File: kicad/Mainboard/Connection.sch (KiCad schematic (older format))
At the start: 12 parts, among them J12 GPS_CONN, J13 DBG_CONN, J15 Micro_SD_Card

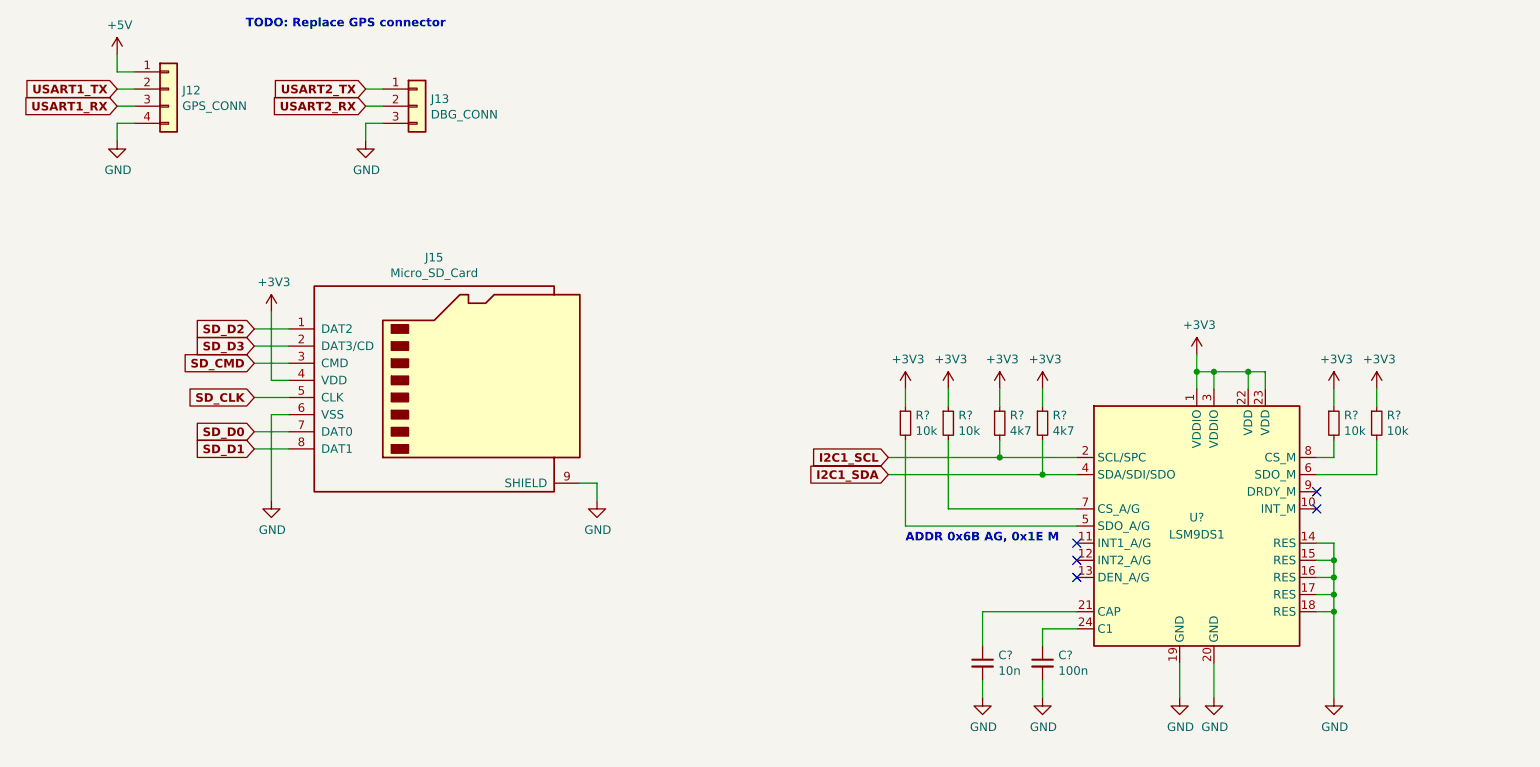
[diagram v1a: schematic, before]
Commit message: Add files via upload
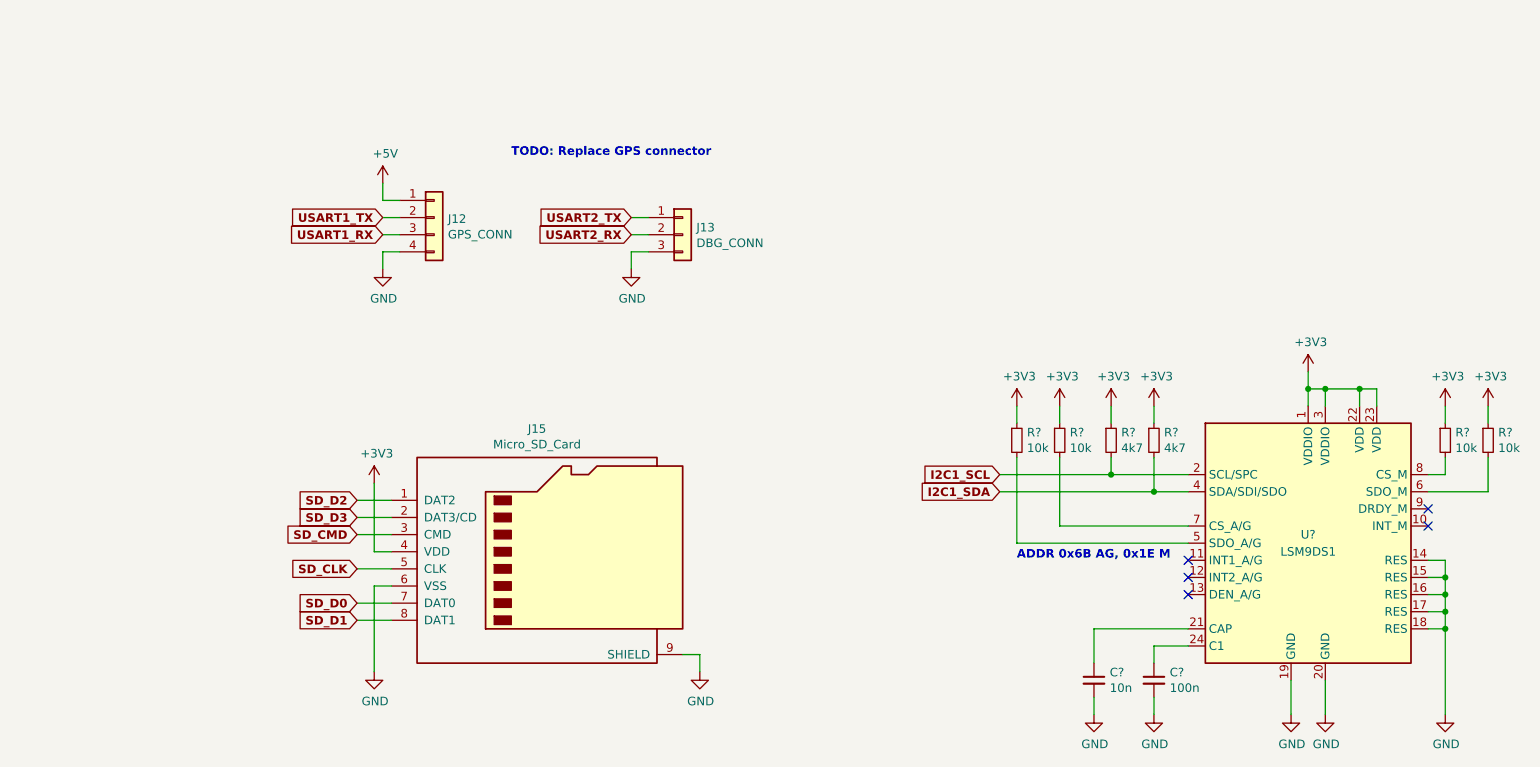
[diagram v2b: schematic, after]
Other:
- moved on the sheet: C?, J12, J13, J15, R?, U?

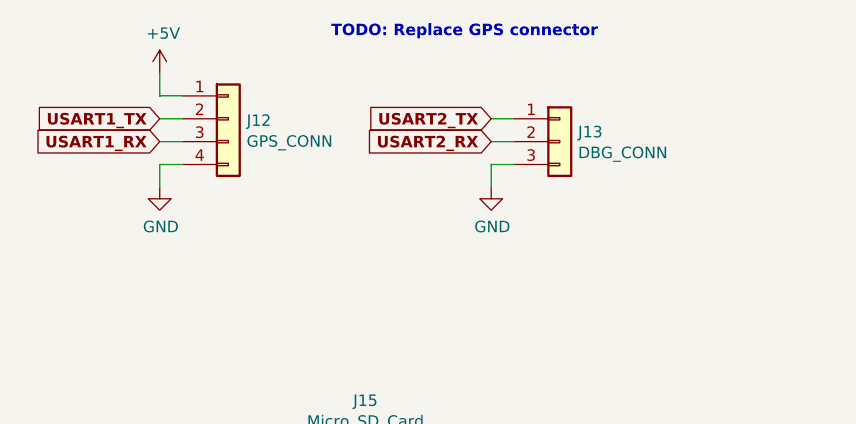
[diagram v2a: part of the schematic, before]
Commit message: Add files via upload
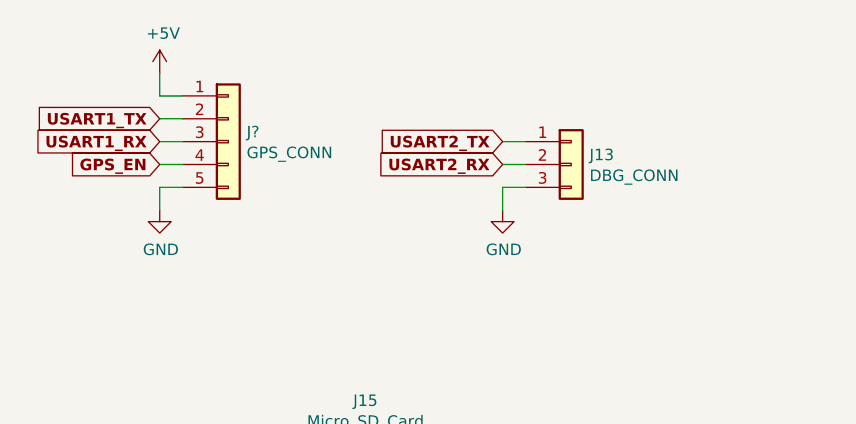
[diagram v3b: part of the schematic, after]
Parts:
- removed J12: GPS_CONN, symbol Mainboard-rescue:Conn_01x04-conn
- added J?: GPS_CONN, symbol Connector_Generic:Conn_01x05
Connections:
- net +5V: now also J?.1 (Pin_1)
- net GND: now also J?.5 (Pin_5)
- net USART1_RX: now also J?.3 (Pin_3)
- net USART1_TX: now also J?.2 (Pin_2)
- new net GPS_EN: J?.4 (Pin_4)
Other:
- note removed: "TODO: Replace GPS connector"
- moved on the sheet: J13
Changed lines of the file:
@@
 $Descr A4 11693 8268
 encoding utf-8
-Sheet 7 7
+Sheet 7 8
 Title "Connections"
 Date ""
@@
 $EndDescr
 $Comp
-L Mainboard-rescue:Conn_01x04-conn J12
-U 1 1 5E07BAA3
-P 3300 1950
-F 0 "J12" H 3380 1942 50  0000 L CNN
-F 1 "GPS_CONN" H 3380 1851 50  0000 L CNN
-F 2 "" H 3300 1950 50  0001 C CNN
-F 3 "~" H 3300 1950 50  0001 C CNN
-	1    3300 1950
-	1    0    0    -1
-$EndComp
-$Comp
 L power:+5V #PWR0104
 U 1 1 5E07BDC5
@@
 L power:GND #PWR0106
 U 1 1 5E07C3FA
-P 3000 2250
-F 0 "#PWR0106" H 3000 2000 50  0001 C CNN
-F 1 "GND" H 3005 2077 50  0000 C CNN
-F 2 "" H 3000 2250 50  0001 C CNN
-F 3 "" H 3000 2250 50  0001 C CNN
-	1    3000 2250
-	1    0    0    -1
-$EndComp
-Wire Wire Line
-	3000 2250 3000 2150
-Wire Wire Line
-	3000 2150 3100 2150
+P 3000 2350
+F 0 "#PWR0106" H 3000 2100 50  0001 C CNN
+F 1 "GND" H 3005 2177 50  0000 C CNN
+F 2 "" H 3000 2350 50  0001 C CNN
+F 3 "" H 3000 2350 50  0001 C CNN
+	1    3000 2350
+	1    0    0    -1
+$EndComp
+Wire Wire Line
+	3000 2350 3000 2250
+Wire Wire Line
+	3000 2250 3100 2250
 Wire Wire Line
 	3100 1950 3000 1950
@@
 L Mainboard-rescue:Conn_01x03-conn J13
 U 1 1 5E07CB74
-P 4750 2050
-F 0 "J13" H 4830 2092 50  0000 L CNN
-F 1 "DBG_CONN" H 4830 2001 50  0000 L CNN
-F 2 "" H 4750 2050 50  0001 C CNN
-F 3 "~" H 4750 2050 50  0001 C CNN
-	1    4750 2050
-	1    0    0    -1
-$EndComp
-Text GLabel 4450 1950 0    50   Input ~ 10
+P 4800 2150
+F 0 "J13" H 4880 2192 50  0000 L CNN
+F 1 "DBG_CONN" H 4880 2101 50  0000 L CNN
+F 2 "" H 4800 2150 50  0001 C CNN
+F 3 "~" H 4800 2150 50  0001 C CNN
+	1    4800 2150
+	1    0    0    -1
+$EndComp
+Text GLabel 4500 2050 0    50   Input ~ 10
 USART2_TX
-Text GLabel 4450 2050 0    50   Input ~ 10
+Text GLabel 4500 2150 0    50   Input ~ 10
 USART2_RX
 $Comp
 L power:GND #PWR0107
 U 1 1 5E07D3F6
-P 4450 2250
-F 0 "#PWR0107" H 4450 2000 50  0001 C CNN
-F 1 "GND" H 4455 2077 50  0000 C CNN
-F 2 "" H 4450 2250 50  0001 C CNN
-F 3 "" H 4450 2250 50  0001 C CNN
-	1    4450 2250
-	1    0    0    -1
-$EndComp
-Wire Wire Line
-	4450 2250 4450 2150
-Wire Wire Line
-	4450 2150 4550 2150
-Wire Wire Line
-	4450 2050 4550 2050
-Wire Wire Line
-	4450 1950 4550 1950
+P 4500 2350
+F 0 "#PWR0107" H 4500 2100 50  0001 C CNN
+F 1 "GND" H 4505 2177 50  0000 C CNN
+F 2 "" H 4500 2350 50  0001 C CNN
+F 3 "" H 4500 2350 50  0001 C CNN
+	1    4500 2350
+	1    0    0    -1
+$EndComp
+Wire Wire Line
+	4500 2350 4500 2250
+Wire Wire Line
+	4500 2250 4600 2250
+Wire Wire Line
+	4500 2150 4600 2150
+Wire Wire Line
+	4500 2050 4600 2050
 $Comp
 L Mainboard-rescue:Micro_SD_Card-conn J15
@@
 Text Notes 6700 3950 0    50   ~ 10
 ADDR 0x6B AG, 0x1E M
-Text Notes 3750 1600 0    50   ~ 10
-TODO: Replace GPS connector
 $Comp
 L Sensor_Motion:LSM9DS1 U?
@@
 Wire Wire Line
 	6600 3550 7500 3550
+$Comp
+L Connector_Generic:Conn_01x05 J?
+U 1 1 5E3E7A55
+P 3300 2050
+F 0 "J?" H 3380 2092 50  0000 L CNN
+F 1 "GPS_CONN" H 3380 2001 50  0000 L CNN
+F 2 "" H 3300 2050 50  0001 C CNN
+F 3 "~" H 3300 2050 50  0001 C CNN
+	1    3300 2050
+	1    0    0    -1
+$EndComp
+Wire Wire Line
+	3000 2150 3100 2150
+Text GLabel 3000 2150 0    50   Input ~ 10
+GPS_EN
 $EndSCHEMATC
